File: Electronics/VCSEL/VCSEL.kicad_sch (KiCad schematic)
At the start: 10 parts, among them J1 Conn_01x06

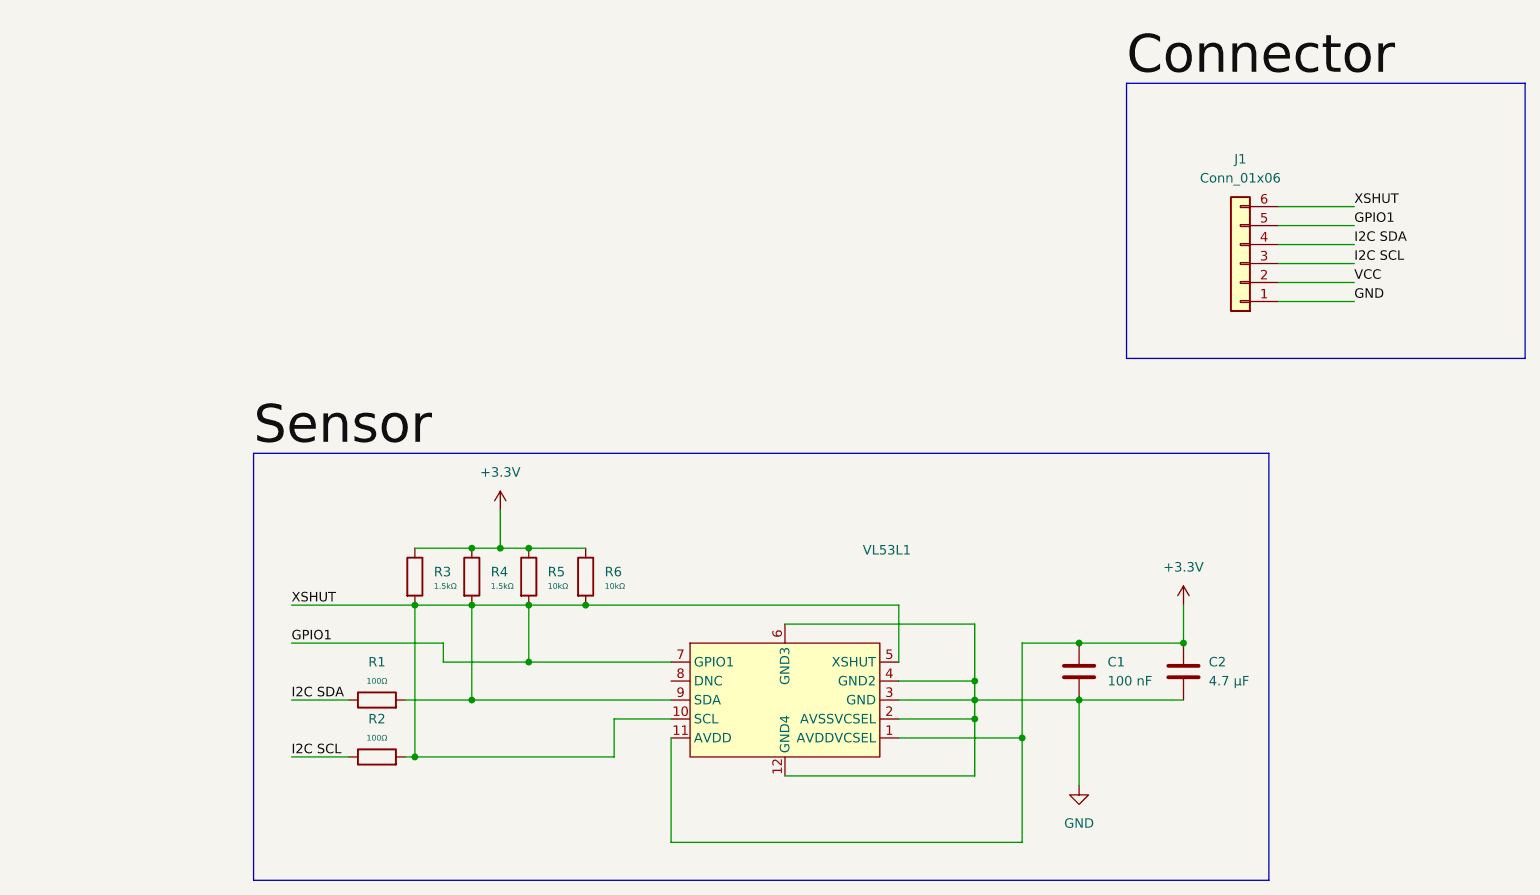
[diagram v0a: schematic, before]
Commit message: V01 VCSEL PCB added
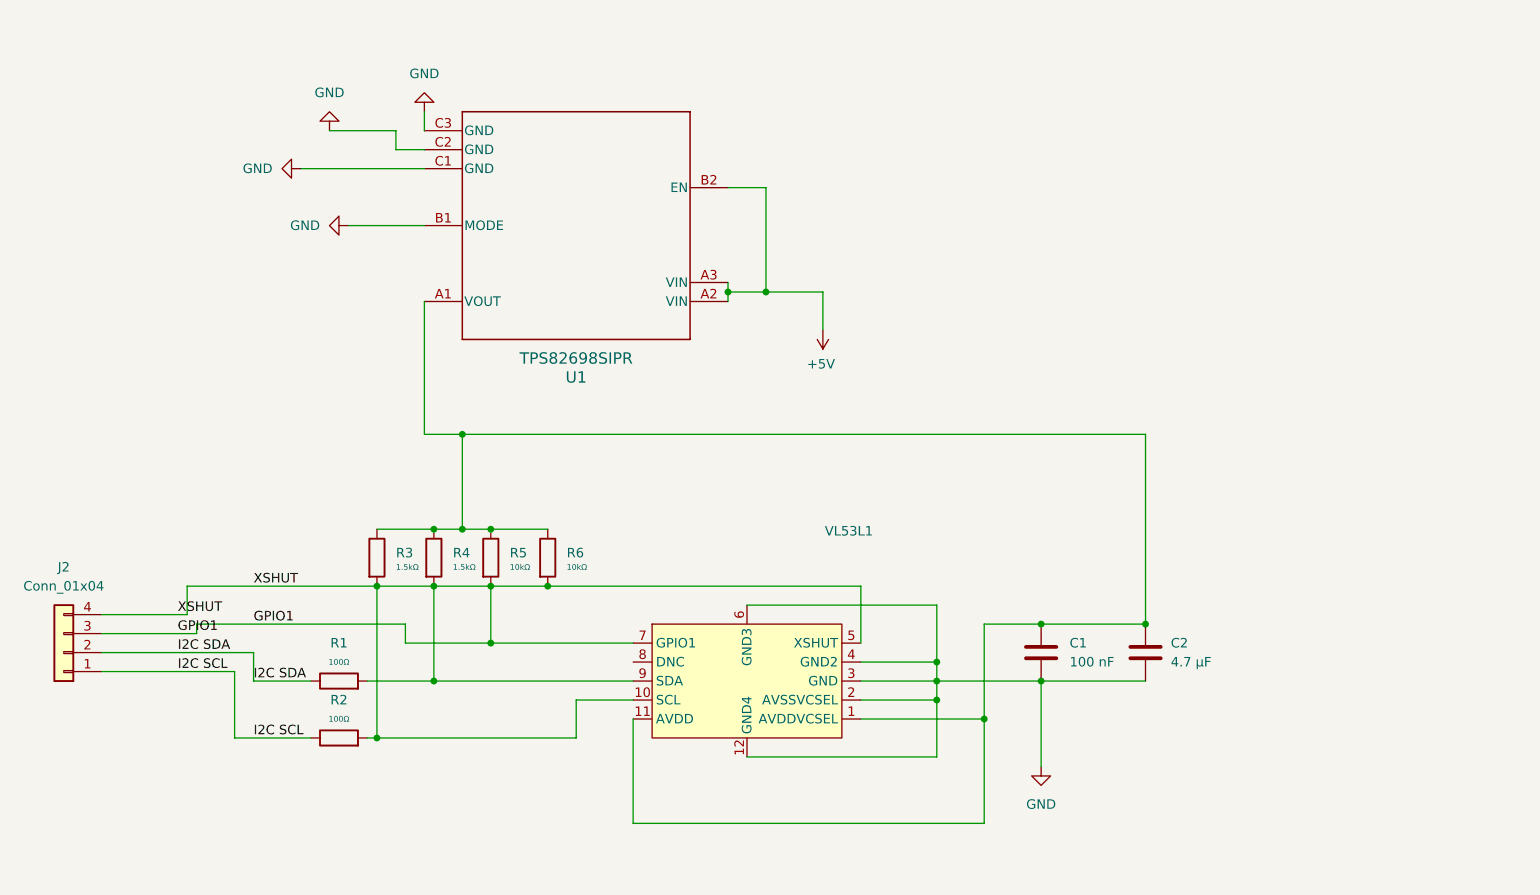
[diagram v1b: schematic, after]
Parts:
- removed J1: Conn_01x06, symbol Connector_Generic:Conn_01x06
- added J2: Conn_01x04, Connector_JST:JST_EH_B4B-EH-A_1x04_P2.50mm_Vertical, symbol Connector_Generic:Conn_01x04
- added U1: TPS82698SIPR, footprints:SIP0008A, symbol 2024-11-04_05-34-17:TPS82698SIPR
- C1, C2: footprint (none) -> Capacitor_SMD:C_0402_1005Metric
- R1, R2, R5, R6: footprint (none) -> Resistor_SMD:R_0402_1005Metric
- R3, R4: footprint (none) -> Resistor_SMD:R_01005_0402Metric
- VL53L1: footprint (none) -> VCSEL_footprints:QFN_BV0FY&slash_1_STM
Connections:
- net GND: now also U1.B1 (MODE), U1.C1 (GND), U1.C2 (GND), U1.C3 (GND)
- net GPIO1: now also J2.3 (Pin_3), J2.4 (Pin_4)
- net I2C SCL: now also J2.1 (Pin_1)
- net I2C SDA: now also J2.2 (Pin_2)
- net +3.3V: no longer names the net of C1.1, C2.1, R3.1, R4.1, R5.1, R6.1, VL53L1.1 (AVDDVCSEL), VL53L1.11 (AVDD)
- net +3.3V: now also U1.A1 (VOUT)
- new net +5V: U1.A2 (VIN), U1.A3 (VIN), U1.B2 (EN)
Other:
- company: (none) -> Georgia Tech Propulsive Landers
- title: (none) -> VCSEL - VL53L1
- moved on the sheet: C1, C2, R1, R2, R3, R4, R5, R6, VL53L1
